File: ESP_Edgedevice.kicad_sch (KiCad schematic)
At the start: 2 parts, among them J1 Screw_Terminal_01x03, U1 ESP32_NODEMCU

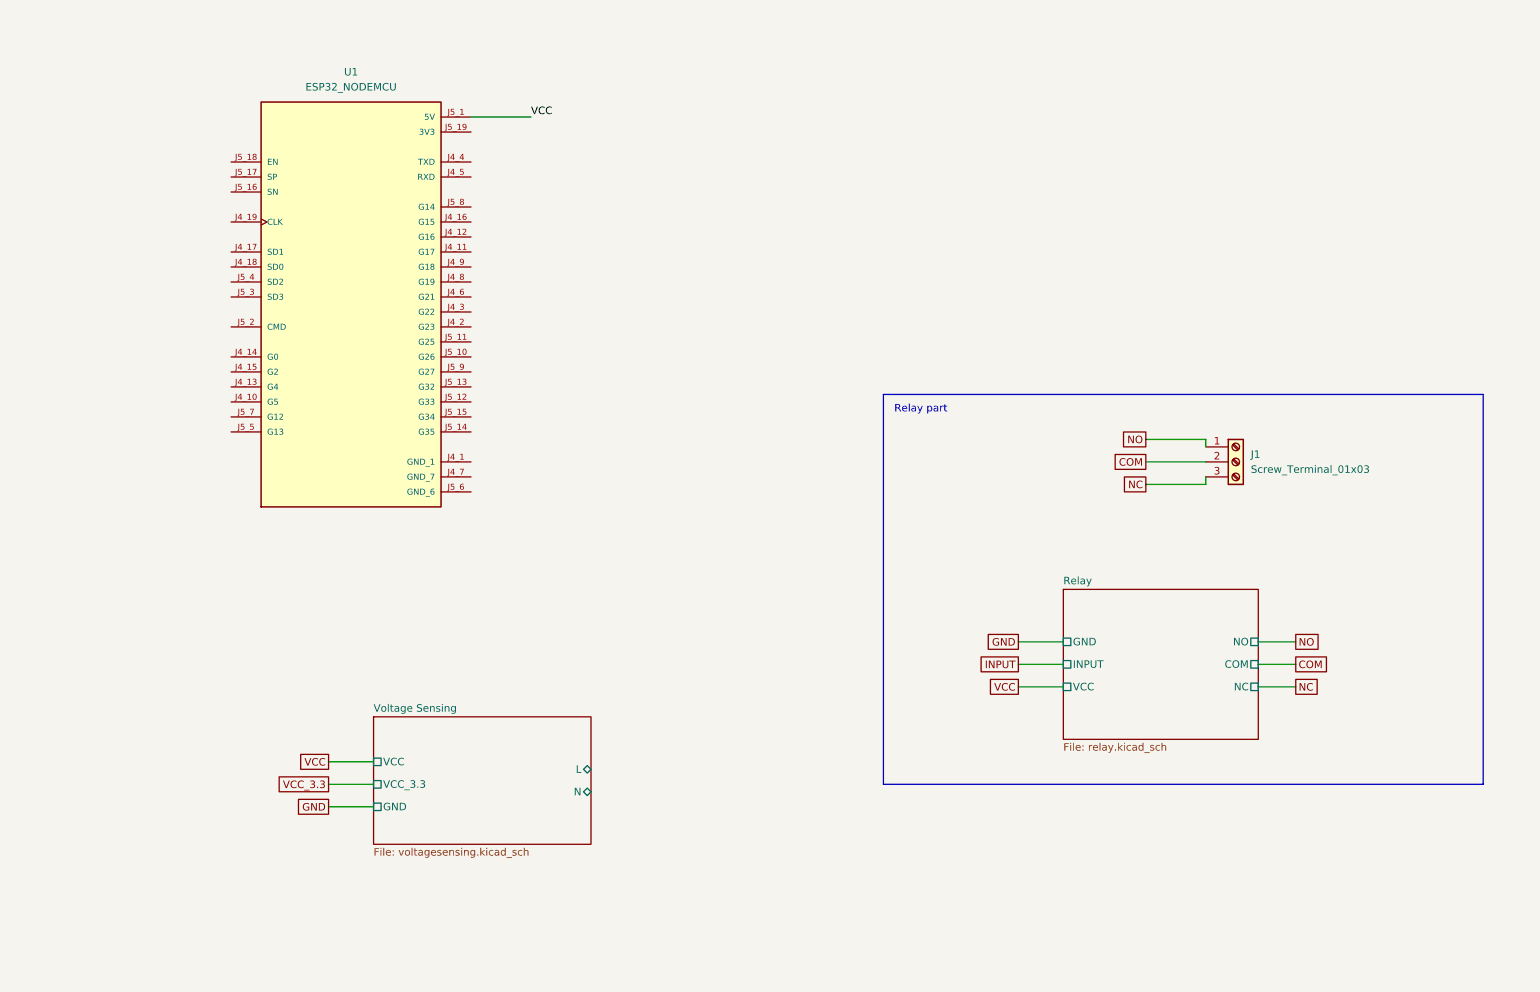
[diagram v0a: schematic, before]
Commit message: minor changes
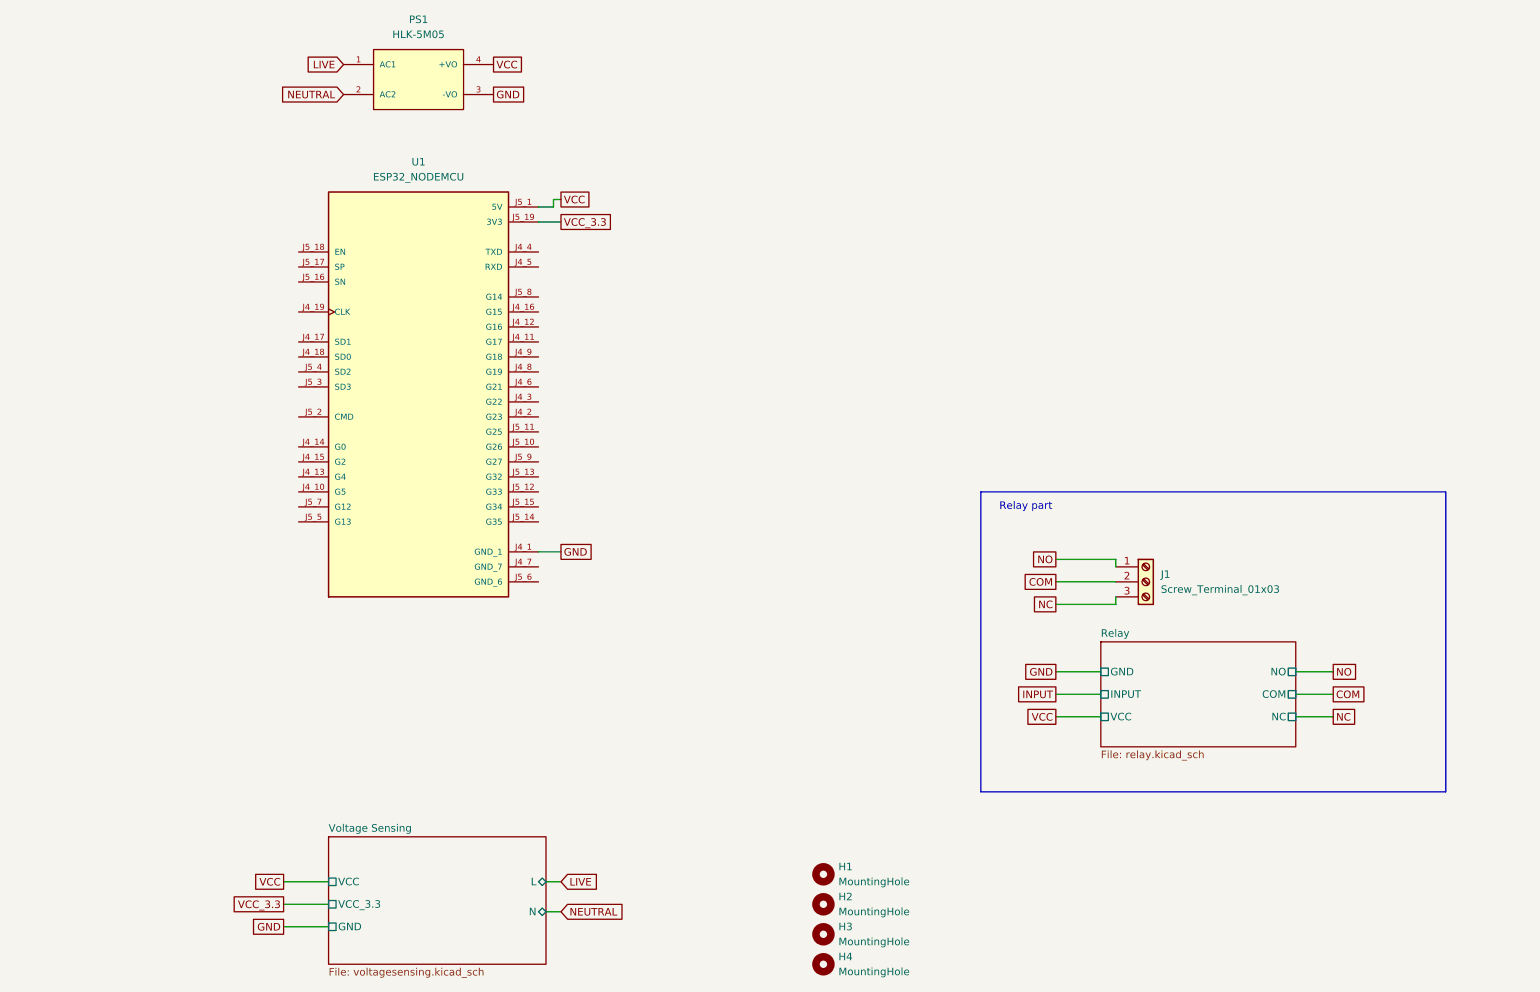
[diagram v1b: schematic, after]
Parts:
- added H1, H2, H3, H4: MountingHole, symbol Mechanical:MountingHole
- added PS1: HLK-5M05, HLK-5M05:CONV_HLK-5M05, symbol HLK-5M05:HLK-5M05
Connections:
- net GND: now also U1.J4_1 (GND_1), PS1.3 (-VO)
- net VCC: now also PS1.4 (+VO)
- net VCC_3.3: now also U1.J5_19 (3V3)
- new net LIVE: PS1.1 (AC1)
- new net NEUTRAL: PS1.2 (AC2)
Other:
- moved on the sheet: J1, U1

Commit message: Final Schematic Editing Completed
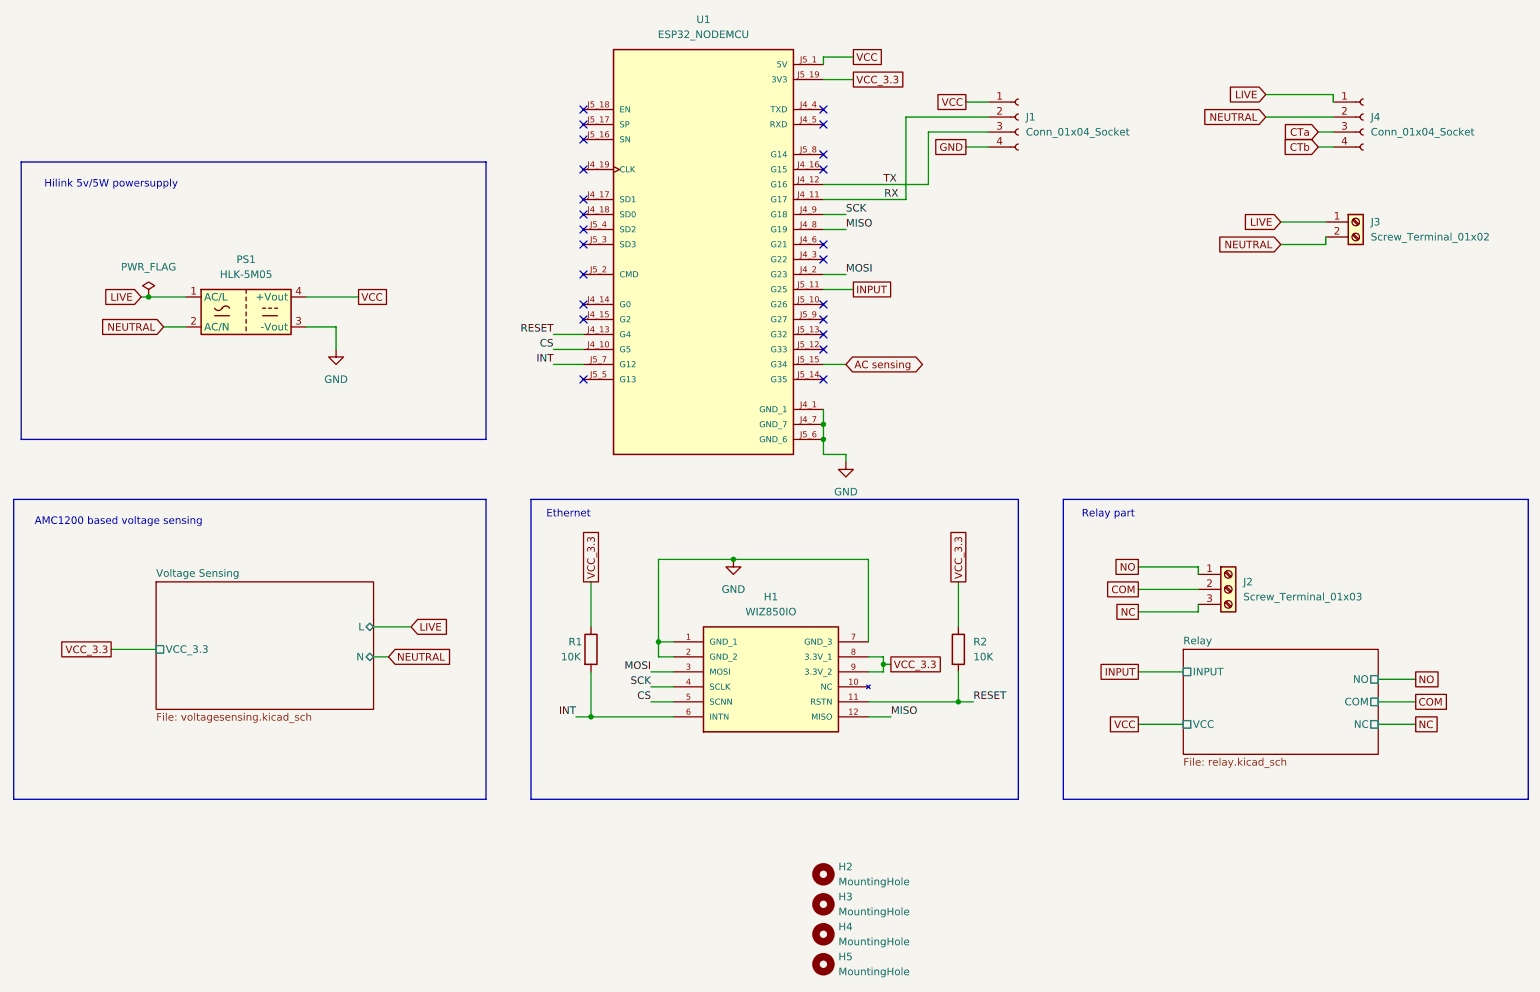
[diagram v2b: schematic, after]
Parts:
- removed PS1: HLK-5M05, HLK-5M05:CONV_HLK-5M05, symbol HLK-5M05:HLK-5M05
- added H1: WIZ850IO, WIZ850IO:WIZ850IO, symbol WIZ850IO:WIZ850IO
- added J1, J4: Conn_01x04_Socket, symbol Connector:Conn_01x04_Socket
- added J3: Screw_Terminal_01x02, symbol Connector:Screw_Terminal_01x02
- added PS1: HLK-5M05, Converter_ACDC:Converter_ACDC_Hi-Link_HLK-5Mxx, symbol Converter_ACDC:HLK-5M05
- added R1, R2: 10K, symbol Device:R
- renumbered H1 to H2, H2 to H3, H3 to H4, H4 to H5, J1 to J2
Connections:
- net GND: now also U1.J4_7 (GND_7), U1.J5_6 (GND_6), H1.1 (GND_1), H1.2 (GND_2), H1.7 (GND_3), J1.4 (Pin_4), PS1.3 (-Vout)
- net INPUT: now also U1.J5_11 (G25)
- net LIVE: now also J3.1 (Pin_1), J4.1 (Pin_1), PS1.1 (AC/L)
- net NEUTRAL: now also J3.2 (Pin_2), J4.2 (Pin_2), PS1.2 (AC/N)
- net VCC: now also J1.1 (Pin_1), PS1.4 (+Vout)
- net VCC_3.3: now also H1.8 (3.3V_1), H1.9 (3.3V_2), R1.1, R2.1
- net CS: now reaches U1.J4_10 (G5)
- net CS: now also H1.5 (SCNN)
- net RX: now reaches U1.J4_11 (G17)
- net RX: now also J1.2 (Pin_2)
- net TX: now reaches U1.J4_12 (G16)
- net TX: now also J1.3 (Pin_3)
- net RESET: now reaches U1.J4_13 (G4)
- net RESET: now also H1.11 (RSTN), R2.2
- net MOSI: now reaches U1.J4_2 (G23)
- net MOSI: now also H1.3 (MOSI)
- net MISO: now reaches U1.J4_8 (G19)
- net MISO: now also H1.12 (MISO)
- net SCK: now reaches U1.J4_9 (G18)
- net SCK: now also H1.4 (SCLK)
- net AC sensing: now reaches U1.J5_15 (G34)
- net INT: now reaches U1.J5_7 (G12)
- net INT: now also H1.6 (INTN), R1.2
- new net CTa: J4.3 (Pin_3)
- new net CTb: J4.4 (Pin_4)
- no-connect marks 0 -> 23
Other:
- sheet Relay ports: added none; removed GND
- sheet Voltage Sensing ports: added none; removed GND, VCC
- note added: "AMC1200 based voltage sensing"
- note added: "Ethernet"
- note added: "Hilink 5v/5W powersupply"
- moved on the sheet: J2
